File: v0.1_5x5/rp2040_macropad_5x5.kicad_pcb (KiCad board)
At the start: 2 copper layers, 86.2 x 70.2 mm, 82 parts, among them J1 USB_C_Receptacle_USB2.0, SW1 KEY_1_00, SW10 KEY_10_21, SW11 KEY_11_22, SW12 KEY_12_23, SW13 SW_SPDT, SW14 KEY_5_04, SW15 KEY_8_13, SW16 MX_LED, SW17 KEY_9_20, SW18 KEY_10_21, SW19 KEY_11_22, SW2 KEY_2_01, SW20 KEY_12_23, SW21 MX_LED, SW22 KEY_9_20, SW23 KEY_10_21, SW24 KEY_11_22, SW25 KEY_12_23, SW26 MX_LED, SW3 KEY_3_02, SW4 KEY_4_03, SW5 KEY_5_10, SW6 KEY_6_11, SW7 KEY_7_12, SW8 KEY_8_13, SW9 KEY_9_20, U1 RP2040, U2 NCP1117-3.3_SOT223, U3 W25Q128JVS, Y1 12MHz

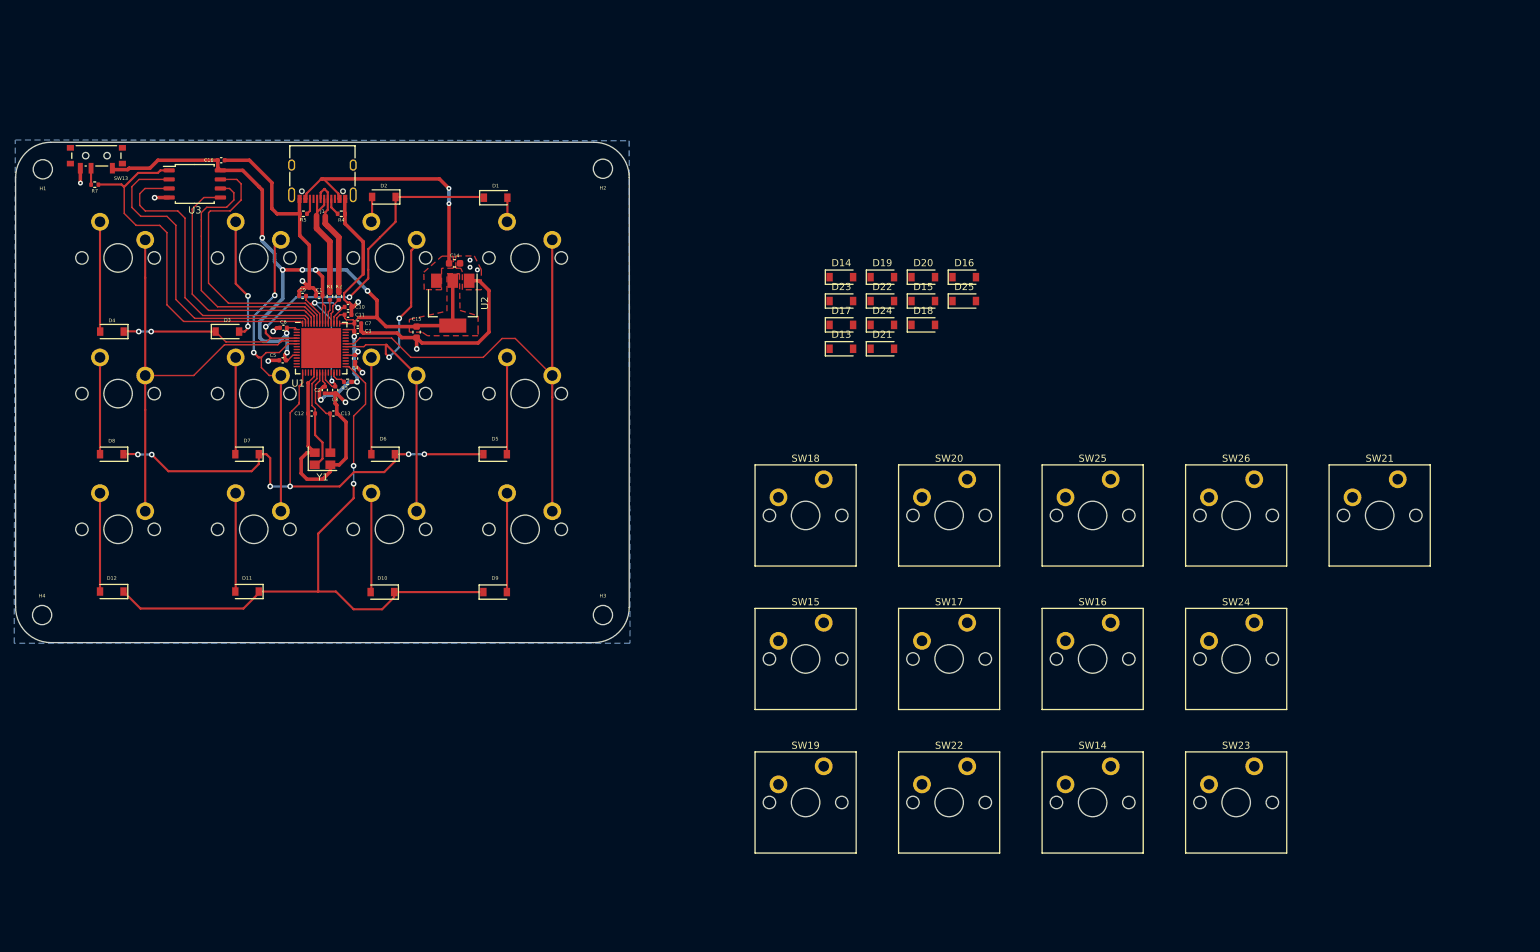
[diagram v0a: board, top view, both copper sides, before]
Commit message: update pcb layout
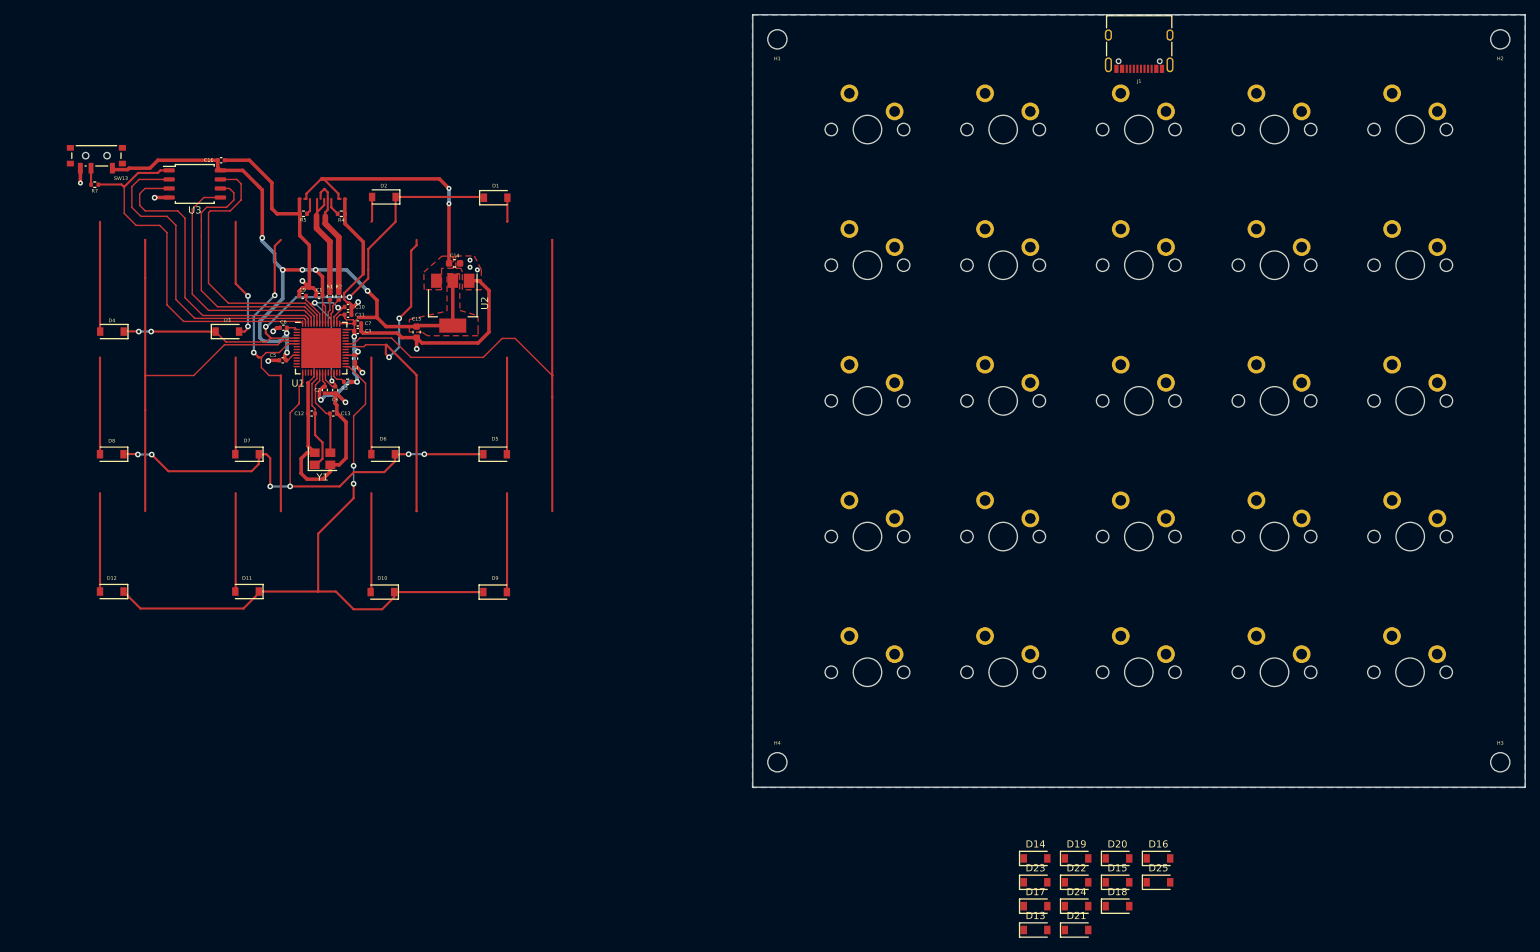
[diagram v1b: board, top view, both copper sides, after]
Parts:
- SW14, SW15, SW16, SW17, SW18, SW19, SW20, SW21, SW22, SW23, SW24, SW25, SW26: moved to B.Cu
- moved SW11 163.4 mm to (240.9, 79.8)
- moved SW12 163.4 mm to (221.8, 79.8)
- moved SW6 144.4 mm to (240.9, 60.7)
- moved SW8 144.4 mm to (202.8, 60.7)
- moved SW7 144.4 mm to (221.8, 60.7)
- moved H3 127.7 mm to (253.5, 130.5)
- moved H2 127.3 mm to (253.5, 29.0)
- moved SW1 125.6 mm to (240.9, 41.7)
- moved SW3 125.6 mm to (202.8, 41.7)
- moved SW2 125.6 mm to (221.8, 41.7)
- moved SW4 125.6 mm to (183.7, 41.7)
- moved J1 116.1 mm to (202.8, 29.5)
- moved H4 105.3 mm to (152.0, 130.5)
- moved H1 104.7 mm to (152.0, 29.0)
- moved D13 86.0 mm to (188.2, 154.1)
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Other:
- board size 86.2 x 70.2 mm -> 108.4 x 108.5 mm
